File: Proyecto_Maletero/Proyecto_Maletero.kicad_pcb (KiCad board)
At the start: 2 copper layers, 65.6 x 60.1 mm, 49 parts, among them J1 DE9_Pins, J2 Conn_01x02, J3 Conn_01x02, J4 Conn_01x03, J5 Conn_01x02, J6 DE9_Pins, J7 Conn_01x04, J9 Conn_01x04, K1 FINDER-34.51, Q2 MMBT5550L, U1 LM1084-5.0, U2 MCP2551-I-SN, U3 PIC18F258-I_SO, U5 LM321, U7 DRV8870DDA, Y1 4MHz

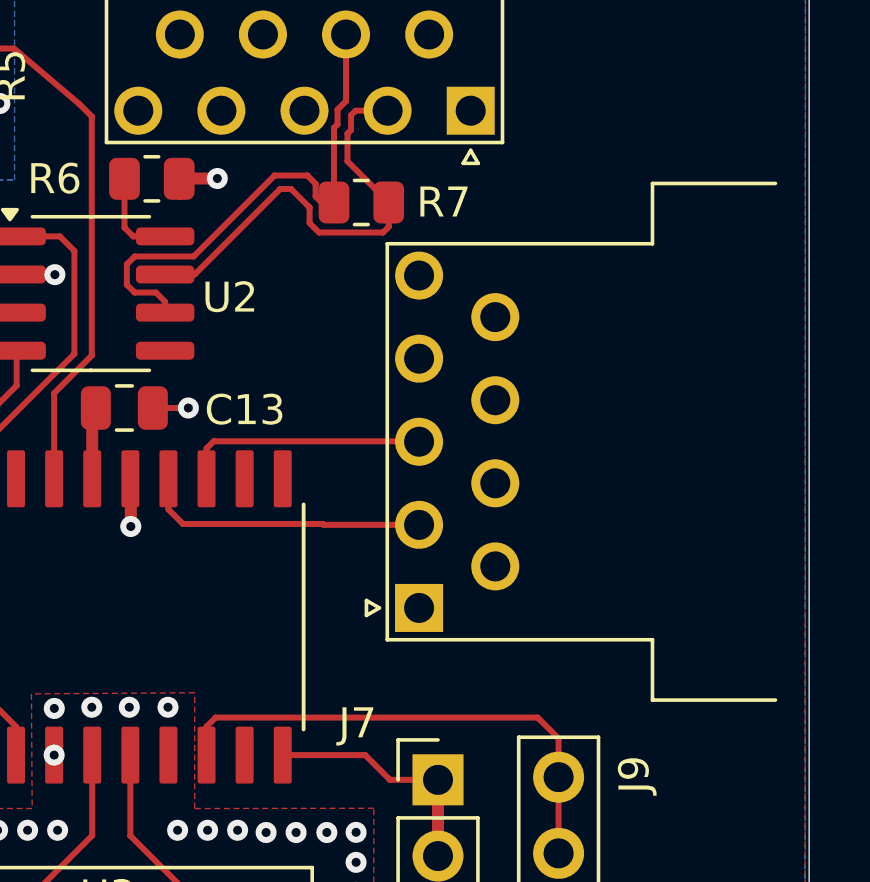
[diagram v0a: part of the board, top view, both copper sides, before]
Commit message: Actulizacion Placa
Mover de9
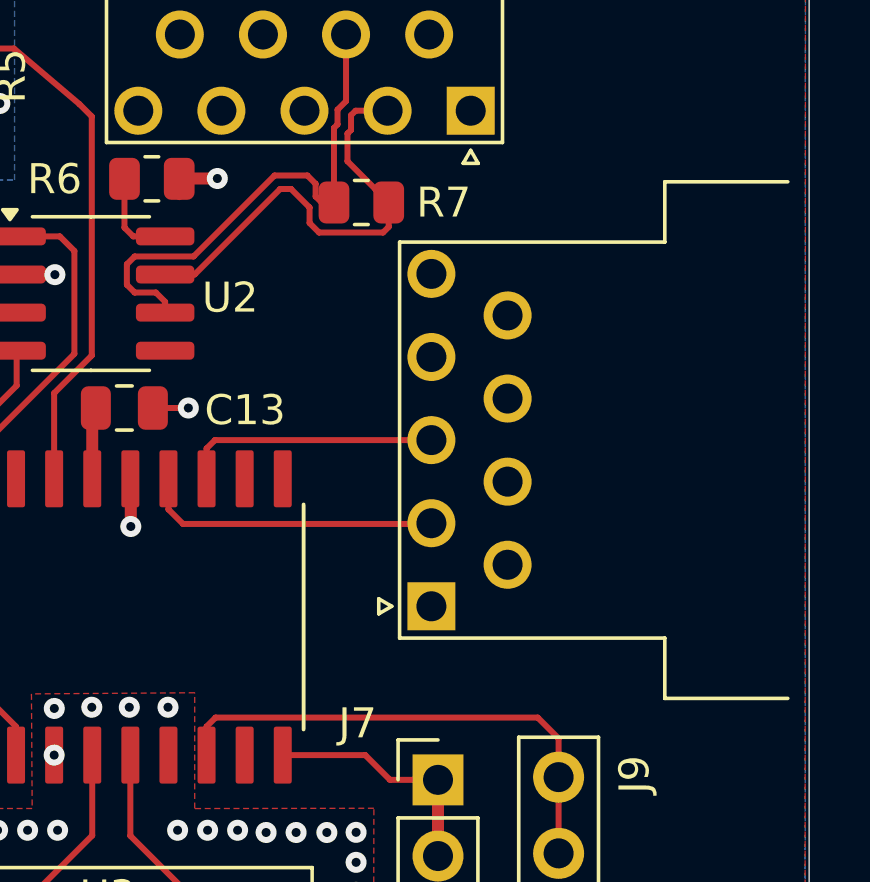
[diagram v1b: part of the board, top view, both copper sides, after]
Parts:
- moved J6 0.41 mm to (161.2, 111.8)
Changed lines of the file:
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@@
 	(footprint "Connector_Dsub:DSUB-9_Pins_Horizontal_P2.77x2.54mm_EdgePinOffset9.40mm"
 		(layer "F.Cu")
-		(at 160.799669 111.84 90)
+		(at 161.21 111.785 90)
 		(descr "9-pin D-Sub connector, horizontal/angled (90 deg), THT-mount, pins (male), pitch 2.77x2.54mm, pin-PCB-offset 9.4mm, see https://docs.rs-online.com/02d6/0900766b81585df2.pdf")
 		(tags "9-pin D-Sub connector horizontal angled 90deg THT pins pitch 2.77x2.54mm pin-PCB-offset 9.4mm")
@@
 	)
 	(segment
-		(start 157.62 109.07)
-		(end 160.799669 109.07)
-		(width 0.2)
-		(layer "F.Cu")
-		(net 16)
-	)
-	(segment
-		(start 157.59 109.04)
-		(end 157.62 109.07)
+		(start 161.185 109.04)
+		(end 152.93 109.04)
 		(width 0.2)
 		(layer "F.Cu")
@@
 	)
 	(segment
-		(start 157.59 109.04)
-		(end 152.93 109.04)
+		(start 152.93 109.04)
+		(end 152.445 108.555)
 		(width 0.2)
 		(layer "F.Cu")
@@
 	)
 	(segment
-		(start 152.93 109.04)
-		(end 152.445 108.555)
+		(start 161.21 109.015)
+		(end 161.185 109.04)
 		(width 0.2)
 		(layer "F.Cu")
@@
 	(segment
 		(start 153.715 106.525)
-		(end 153.715 107.535)
+		(end 153.995 106.245)
 		(width 0.2)
 		(layer "F.Cu")
@@
 	)
 	(segment
-		(start 160.783669 106.284)
-		(end 153.956 106.284)
+		(start 153.995 106.245)
+		(end 161.21 106.245)
 		(width 0.2)
 		(layer "F.Cu")
@@
 	)
 	(segment
-		(start 153.956 106.284)
+		(start 153.715 107.535)
 		(end 153.715 106.525)
 		(width 0.2)
